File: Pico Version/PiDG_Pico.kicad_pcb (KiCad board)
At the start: 2 copper layers, 160 x 99.7 mm, 44 parts, among them J1 Conn_02x05_Odd_Even, J10 Trig, J11 Laser Enable, J12 Pixel Reset, J16 Conn_01x24_Pin, J17 Conn_01x24_Pin, J2 Conn_02x05_Odd_Even, J3 Conn_02x05_Odd_Even, J4 Conn_02x05_Odd_Even, J5 Conn_02x05_Odd_Even, J6 Conn_02x05_Odd_Even, J7 Laser 1, J8 Laser 2, U1 74LVC1G04, U10 74LVC1G08, U11 Teensy4.1, U12 74LVC1G08, U2 SN74LVC04AD, U3 74LVC1G04, U4 SN74LVC04AD, U5 74LVC1G04, U6 SN74LVC04AD, U7 74LVC1G08, U8 74LVC1G08, U9 NCP718xSN180

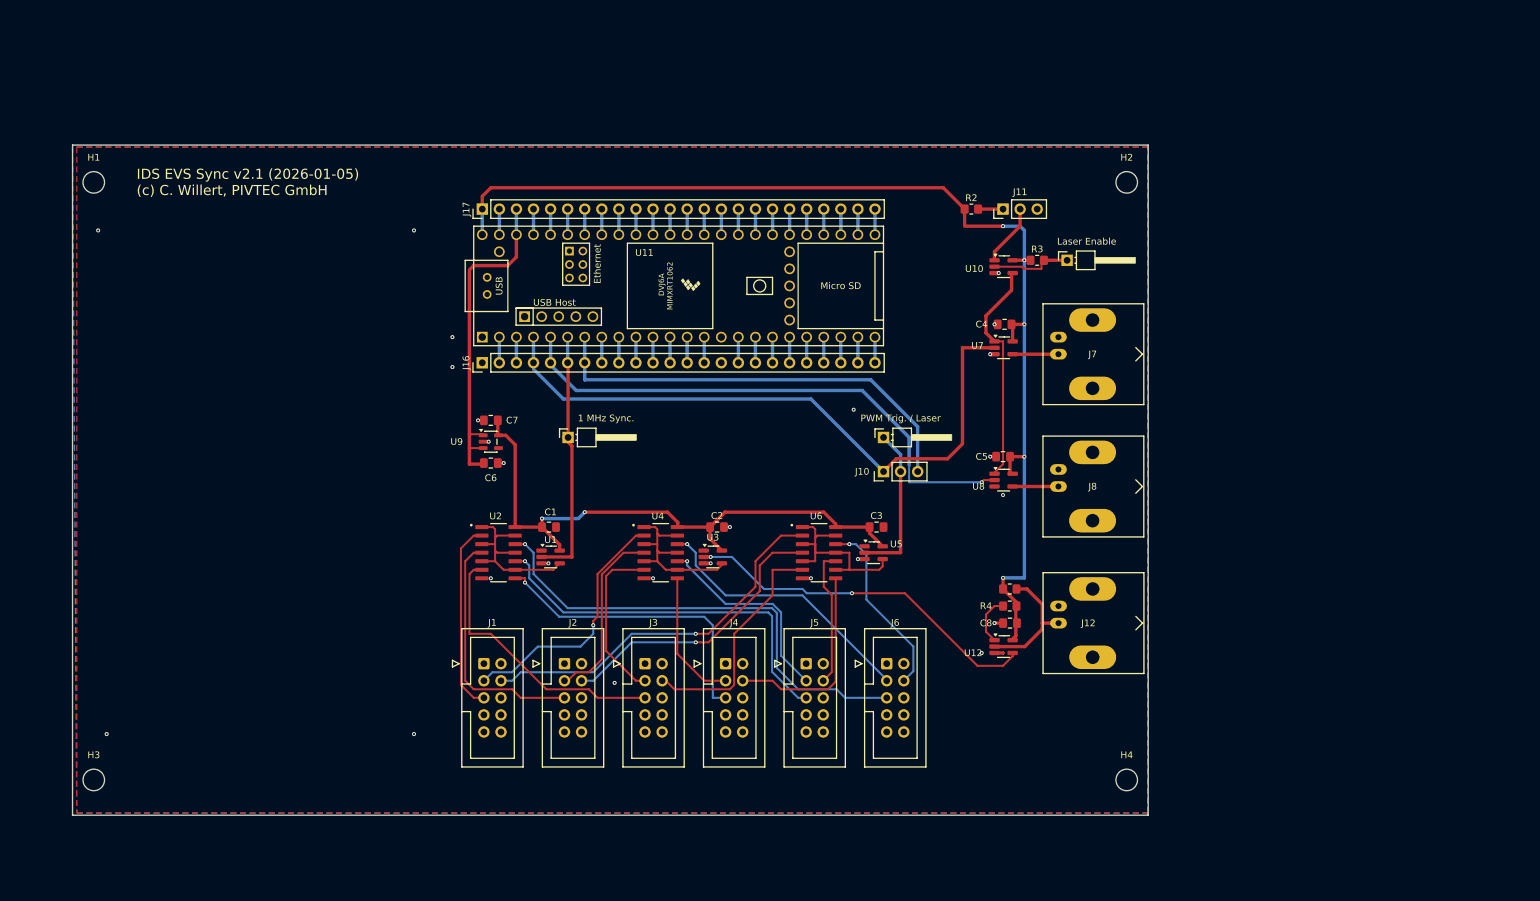
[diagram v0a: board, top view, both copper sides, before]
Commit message: Mor AI workings
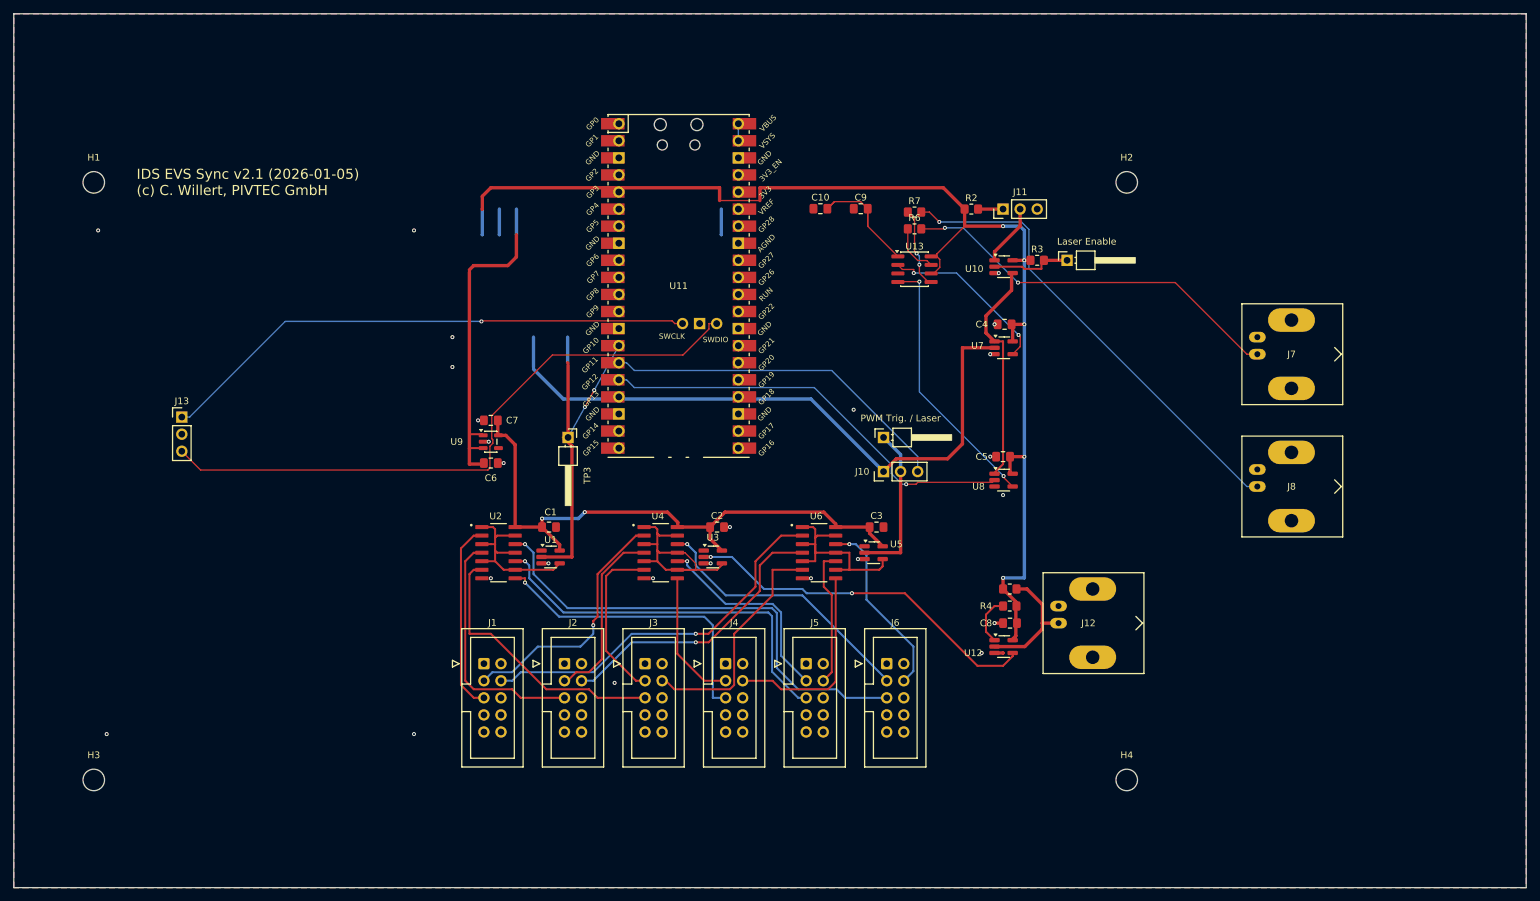
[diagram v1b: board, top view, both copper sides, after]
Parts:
- removed J16, J17: Conn_01x24_Pin, Connector_PinHeader_2.54mm:PinHeader_1x24_P2.54mm_Vertical
- added C10: 1uF, Capacitor_SMD:C_0805_2012Metric_Pad1.18x1.45mm_HandSolder, F.Cu at (190.0, 59.0)
- added C9: 0.1uF, Capacitor_SMD:C_0805_2012Metric_Pad1.18x1.45mm_HandSolder, F.Cu at (196.0, 59.0)
- added J13: Debug, Connector_PinHeader_2.54mm:PinHeader_1x03_P2.54mm_Vertical, F.Cu at (95.0, 90.0)
- added R6: 47, Resistor_SMD:R_0805_2012Metric_Pad1.20x1.40mm_HandSolder, F.Cu at (204.0, 62.0)
- added R7: 47, Resistor_SMD:R_0805_2012Metric_Pad1.20x1.40mm_HandSolder, F.Cu at (204.0, 59.5)
- added U13: UCC27524, Package_SO:SOIC-8_3.9x4.9mm_P1.27mm, F.Cu at (204.0, 68.0)
- TP3: renamed from 1 MHz Sync.
- U11: value Teensy4.1 -> Raspberry Pi Pico 2 W; footprint teensy:Teensy41 -> RPi_Pico:RPi_Pico2W_SMD_TH
- moved J7 29.6 mm to (255.0, 80.6)
- moved J8 29.6 mm to (255.0, 100.3)
- turned TP3 to -90 degrees
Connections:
- net /Pixel reset renamed Pixel reset
- net /Sync1 renamed Net-(J1-Pad5)
- net /Sync2 renamed Net-(J2-Pad5)
- net /Sync3 renamed Net-(J3-Pad5)
- net /Sync4 renamed Net-(J4-Pad5)
- net /Sync5 renamed Sync5
- net /Sync6 renamed Sync6
- net /TDRSTN1 renamed Net-(J1-Pad3)
- net /TDRSTN2 renamed Net-(J2-Pad3)
- net /TDRSTN3 renamed Net-(J3-Pad3)
- net /TDRSTN4 renamed Net-(J4-Pad3)
- net /TDRSTN5 renamed Net-(J5-Pad3)
- net /TDRSTN6 renamed Net-(J6-Pad3)
- net /Trigger 1 renamed Trigger 1
- net /Trigger 2 renamed Trigger 2
- net /Trigger3 renamed Trigger3
- net /Trigger4 renamed Trigger4
- net /Trigger5 renamed Trigger5
- net /Trigger6 renamed Trigger6
- J10 pad 1: /_PULSE_OUT_CH1 -> _PULSE_OUT_CH1
- J10 pad 2: Net-(J10-Pin_2) -> Net-(J10-Pad2)
- J10 pad 3: /PWM_Trig -> PWM_Trig
- J7 pad 1: Net-(J7-In) -> CH1_DRIVE
- J8 pad 1: Net-(J8-In) -> CH2_DRIVE
- TP3 pad 1: /PWM_1MHz -> Net-(TP3-Pad1)
- U1 pad 2: /PWM_1MHz -> Net-(TP3-Pad1)
- U11 pad 1: GND -> (no net)
- U11 pad 10: Net-(J16-Pin_10) -> (no net)
- U11 pad 11: Net-(J16-Pin_11) -> (no net)
- U11 pad 12: Net-(J16-Pin_12) -> (no net)
- U11 pad 13: Net-(J16-Pin_13) -> (no net)
- U11 pad 14: Net-(J16-Pin_14) -> PWM_1MHz
- U11 pad 15: unconnected-(U11-3V3-Pad15) -> PWM_Trig
- U11 pad 16: Net-(J16-Pin_16) -> _PULSE_OUT_CH2
- U11 pad 17: Net-(J16-Pin_17) -> _PULSE_OUT_CH1
- U11 pad 18: Net-(J16-Pin_18) -> GND
- U11 pad 19: Net-(J16-Pin_19) -> (no net)
- U11 pad 2: Net-(J16-Pin_2) -> (no net)
- U11 pad 20: Net-(J16-Pin_20) -> (no net)
- U11 pad 21: Net-(J16-Pin_21) -> (no net)
- U11 pad 22: Net-(J16-Pin_22) -> (no net)
- U11 pad 23: Net-(J16-Pin_23) -> (no net)
- U11 pad 24: Net-(J16-Pin_24) -> (no net)
- U11 pad 25: Net-(J17-Pin_24) -> GND
- U11 pad 26: Net-(J17-Pin_23) -> (no net)
- U11 pad 27: Net-(J17-Pin_22) -> (no net)
- U11 pad 28: Net-(J17-Pin_21) -> (no net)
- U11 pad 29: Net-(J17-Pin_20) -> (no net)
- U11 pad 3: Net-(J16-Pin_3) -> (no net)
- U11 pad 30: Net-(J17-Pin_19) -> (no net)
- U11 pad 31: Net-(J17-Pin_18) -> (no net)
- U11 pad 32: Net-(J17-Pin_17) -> (no net)
- U11 pad 33: Net-(J17-Pin_16) -> (no net)
- U11 pad 34: GND -> (no net)
- U11 pad 35: Net-(J17-Pin_14) -> (no net)
- U11 pad 36: Net-(J17-Pin_13) -> +3V3
- U11 pad 37: Net-(J17-Pin_12) -> (no net)
- U11 pad 38: Net-(J17-Pin_11) -> (no net)
- U11 pad 39: Net-(J17-Pin_10) -> +5V
- U11 pad 4: /_PULSE_OUT_CH1 -> (no net)
- U11 pad 40: Net-(J17-Pin_9) -> +5V
- U11 pad 42: Net-(J17-Pin_7) -> GND
- U11 pad 5: /_PULSE_OUT_CH2 -> (no net)
- U11 pad 6: /PWM_1MHz -> (no net)
- U11 pad 7: /PWM_Trig -> (no net)
- U11 pad 8: Net-(J16-Pin_8) -> (no net)
- U11 pad 9: Net-(J16-Pin_9) -> (no net)
- U5 pad 2: Net-(J10-Pin_2) -> Net-(J10-Pad2)
- U7 pad 2: /_PULSE_OUT_CH1 -> _PULSE_OUT_CH1
- U7 pad 4: Net-(J7-In) -> CH1_GATED
- U8 pad 2: /_PULSE_OUT_CH2 -> _PULSE_OUT_CH2
- U8 pad 4: Net-(J8-In) -> CH2_GATED
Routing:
- net _PULSE_OUT_CH1: track 0.00 -> 95.3 mm
- net /_PULSE_OUT_CH1: track 95.3 -> 0.00 mm
- net Net-(J13-Pad3): track 3.81 -> 94.8 mm
- net /_PULSE_OUT_CH2: track 81.1 -> 0.00 mm, vias 1 -> 0
- net Net-(J13-Pad1): track 3.81 -> 80.6 mm, vias 0 -> 1
- net CH2_DRIVE: track 0.00 -> 70.3 mm, vias 0 -> 1
- net /PWM_Trig: track 65.4 -> 0.00 mm
- net _PULSE_OUT_CH2: track 0.00 -> 63.3 mm, vias 0 -> 1
- net CH1_DRIVE: track 0.00 -> 57.8 mm, vias 0 -> 2
- net PWM_Trig: track 0.00 -> 52.5 mm
- net CH2_GATED: track 0.00 -> 39.4 mm, vias 0 -> 2
- net +5V: track 167.3 -> 205.4 mm
- net Net-(TP3-Pad1): track 0.00 -> 34.0 mm
- net /PWM_1MHz: track 37.5 -> 3.81 mm
- net CH1_GATED: track 0.00 -> 26.0 mm, vias 0 -> 2
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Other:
- board size 160 x 99.7 mm -> 225 x 130 mm
